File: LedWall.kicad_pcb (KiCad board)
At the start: 2 copper layers, 205 x 205 mm, 107 parts, among them J101 Conn_02x05_Odd_Even, J102 Conn_02x05_Odd_Even, J103 Conn_02x05_Odd_Even, J104 Conn_02x05_Odd_Even, U201 TPS5430DDA

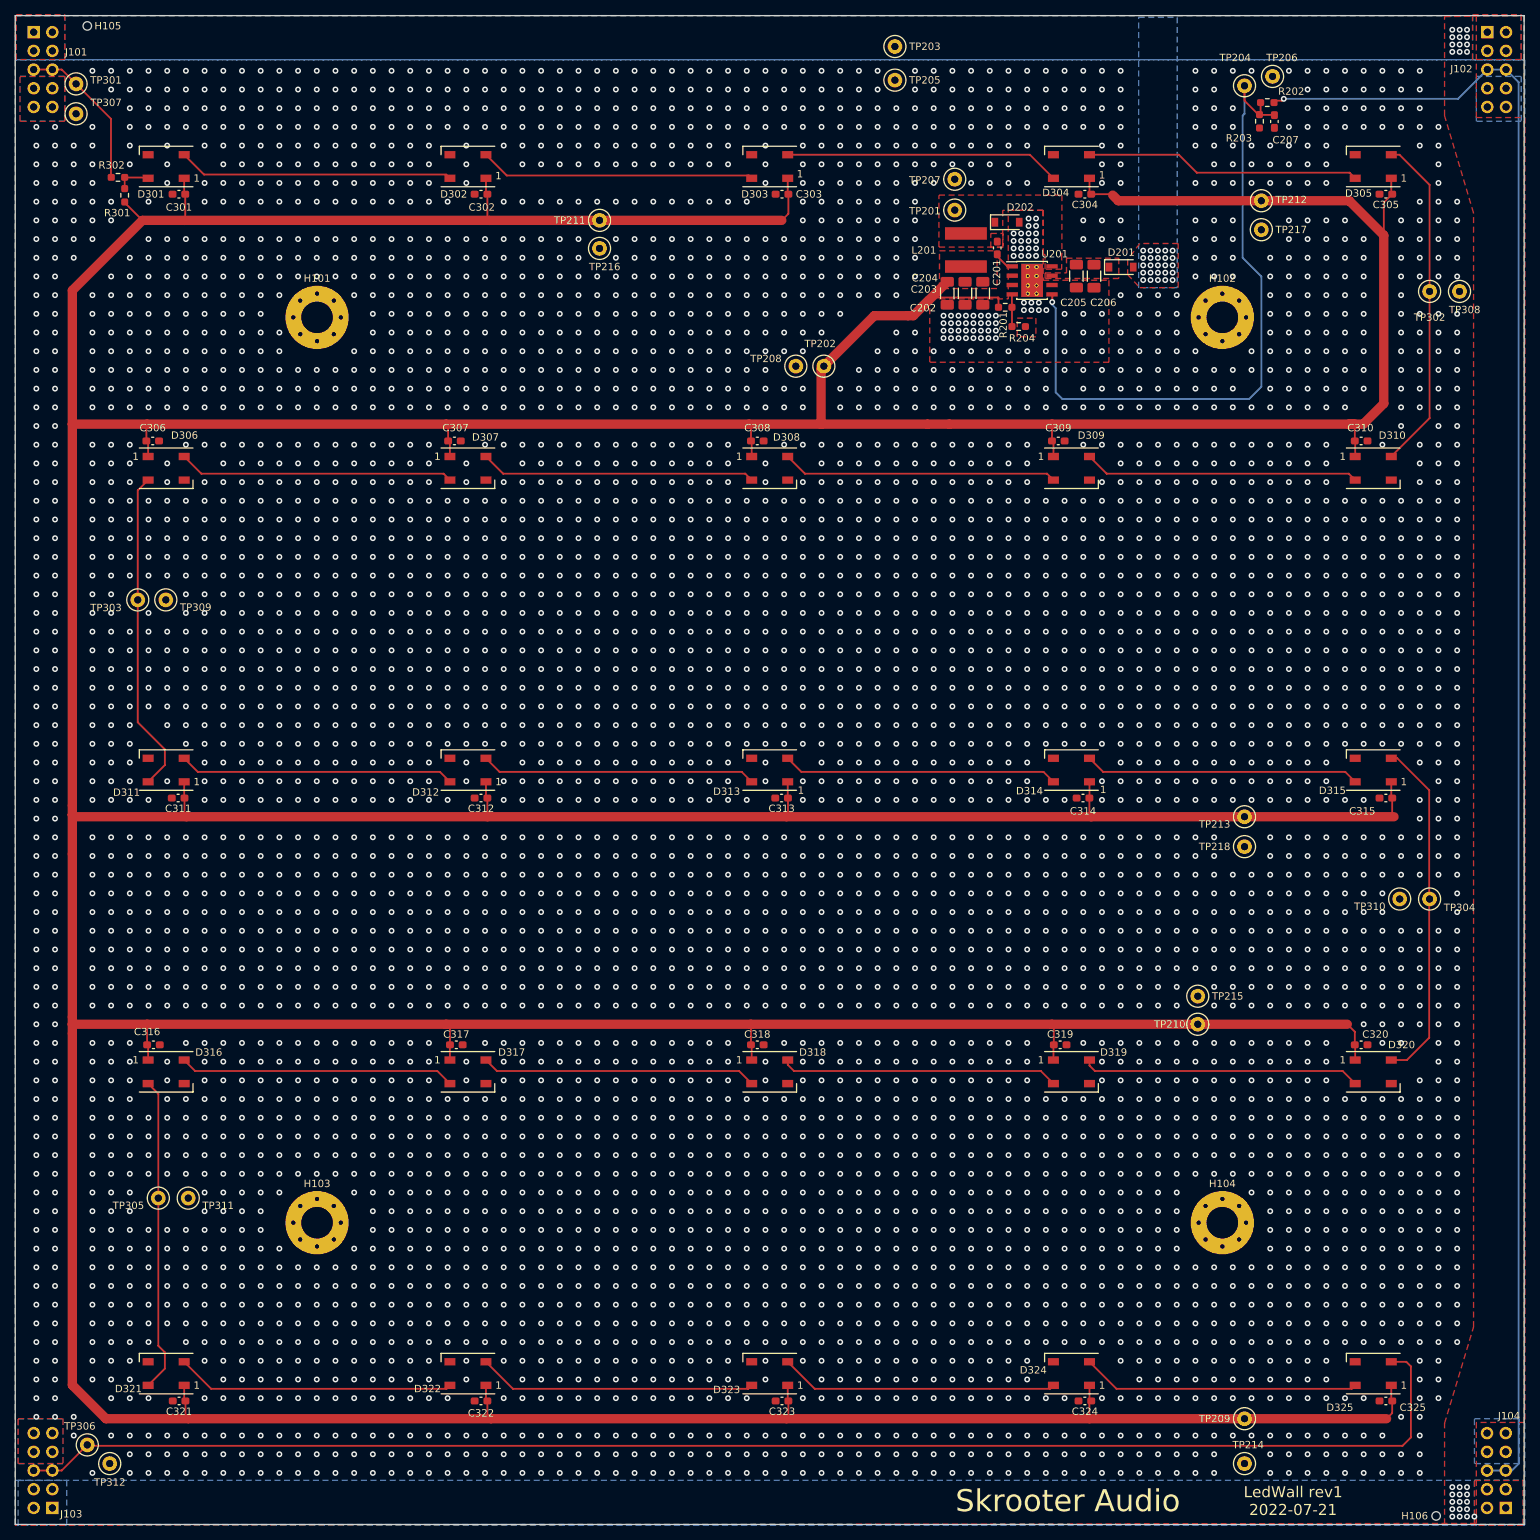
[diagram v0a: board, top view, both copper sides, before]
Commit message: Reduce board size
0.5mm have been removed from all sides
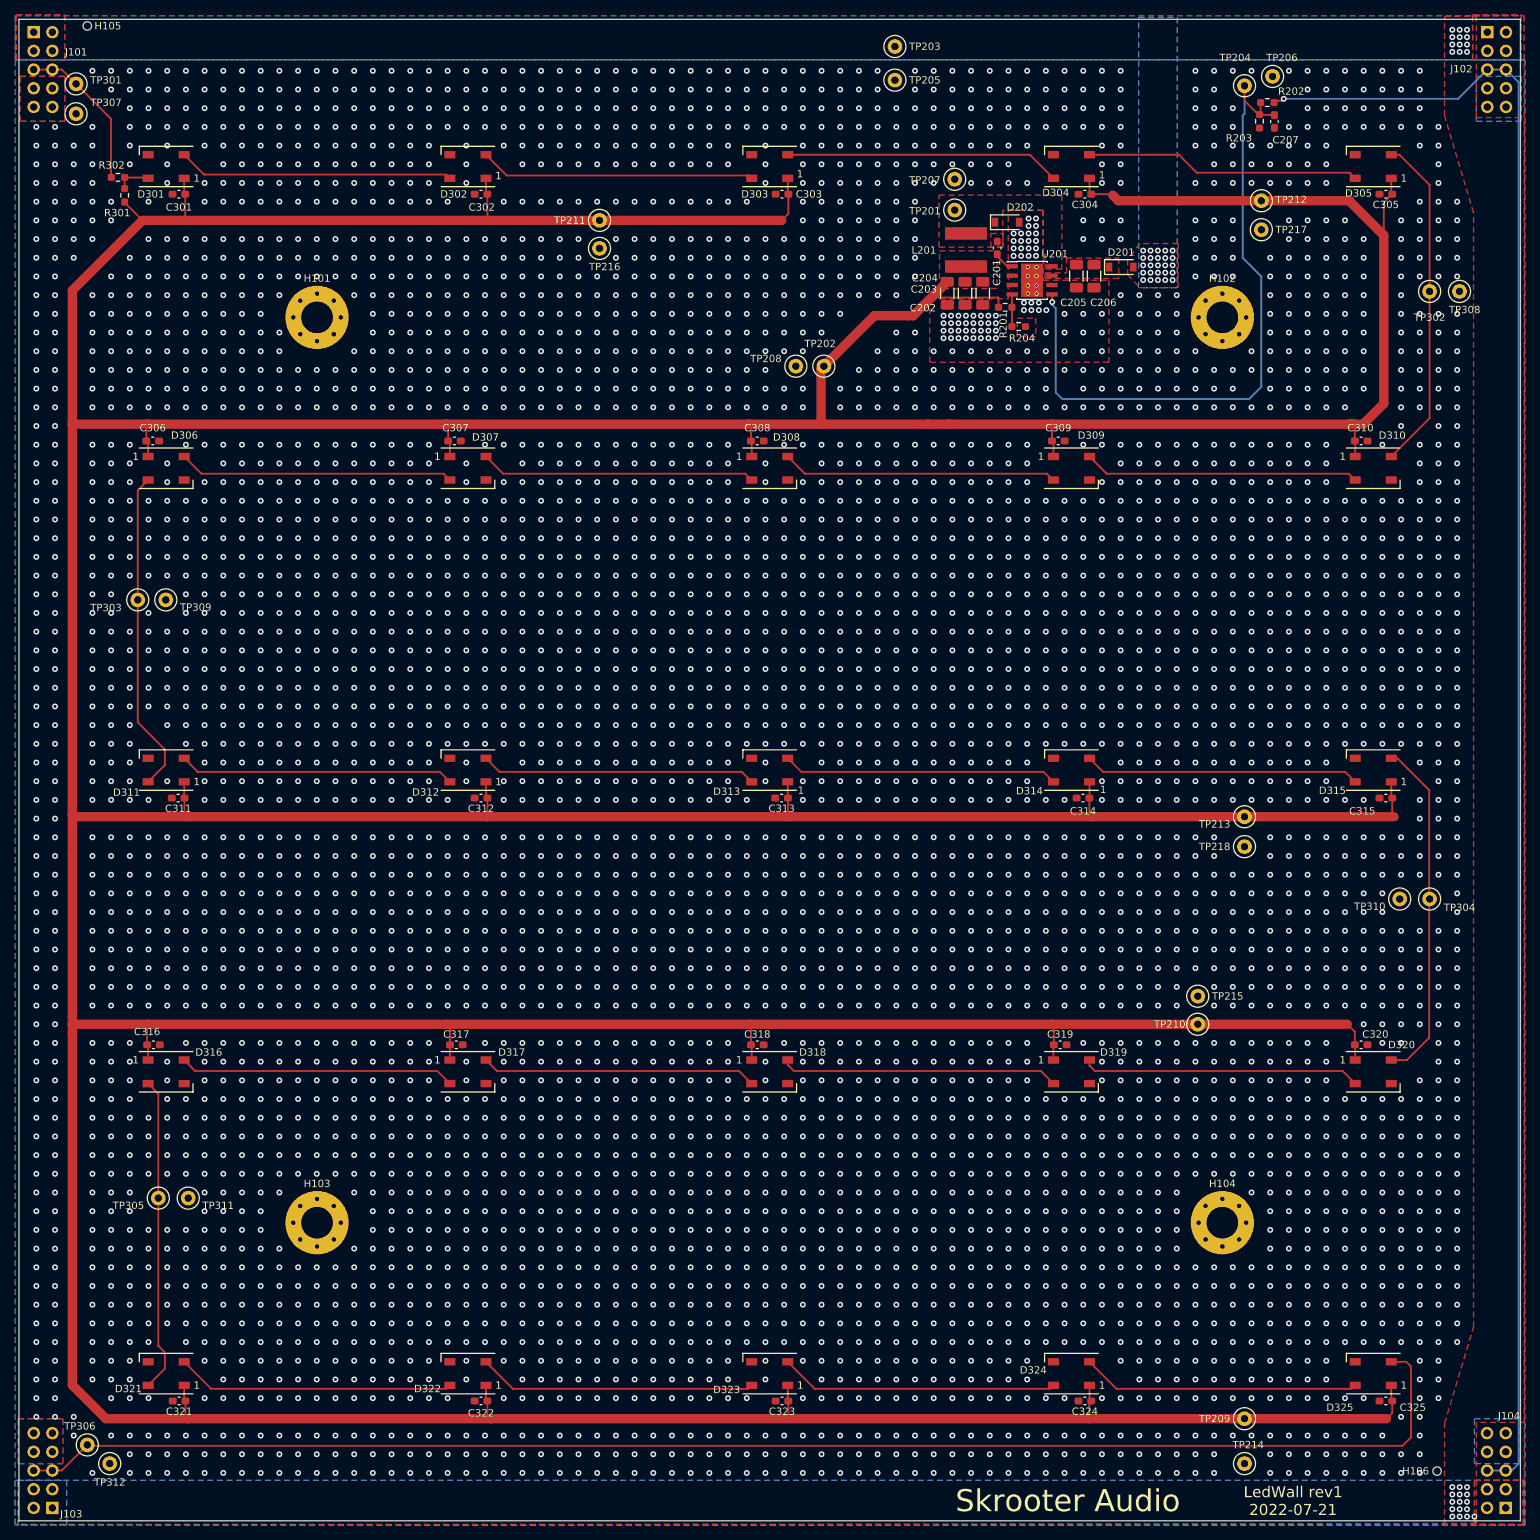
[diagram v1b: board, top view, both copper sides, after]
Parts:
- moved H106 6.10 mm to (233.2, 237.7)
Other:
- board size 205 x 205 mm -> 204 x 204 mm
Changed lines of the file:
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@@
   )
   (footprint "JLC:JLC_toolinghole" (layer "F.Cu")
-    (at 233.045 243.84)
+    (at 233.172 237.744)
     (property "Sheetfile" "File: LedWall.kicad_sch")
     (property "Sheetname" "")
@@
     )
   )
-  (gr_line (start 40 40) (end 40 245) (layer "Edge.Cuts") (width 0.15))
-  (gr_line (start 40 40) (end 245 40) (layer "Edge.Cuts") (width 0.15))
-  (gr_line (start 245 40) (end 245 245) (layer "Edge.Cuts") (width 0.15))
-  (gr_line (start 40 245) (end 245 245) (layer "Edge.Cuts") (width 0.15))
+  (gr_line (start 40.5 40.5) (end 40.5 244.5) (layer "Edge.Cuts") (width 0.15))
+  (gr_line (start 40.5 40.5) (end 244.5 40.5) (layer "Edge.Cuts") (width 0.15))
+  (gr_line (start 244.5 40.5) (end 244.5 244.5) (layer "Edge.Cuts") (width 0.15))
+  (gr_line (start 40.5 244.5) (end 244.5 244.5) (layer "Edge.Cuts") (width 0.15))
   (gr_text "Vin: 12V-36V" (at 227.33 41.656) (layer "B.SilkS")
     (effects (font (size 1 1) (thickness 0.15)) (justify mirror))
